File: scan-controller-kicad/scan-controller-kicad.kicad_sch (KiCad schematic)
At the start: 34 parts, among them CN1 24V in, J3 Raspi GPIO, J4 Raspi UART, J5 ICSP, J6 FTDI, Q6 IRLML2502, Q7 IRLML6402, SW6 Reset, U6 ATmega328P, Y1 8MHz

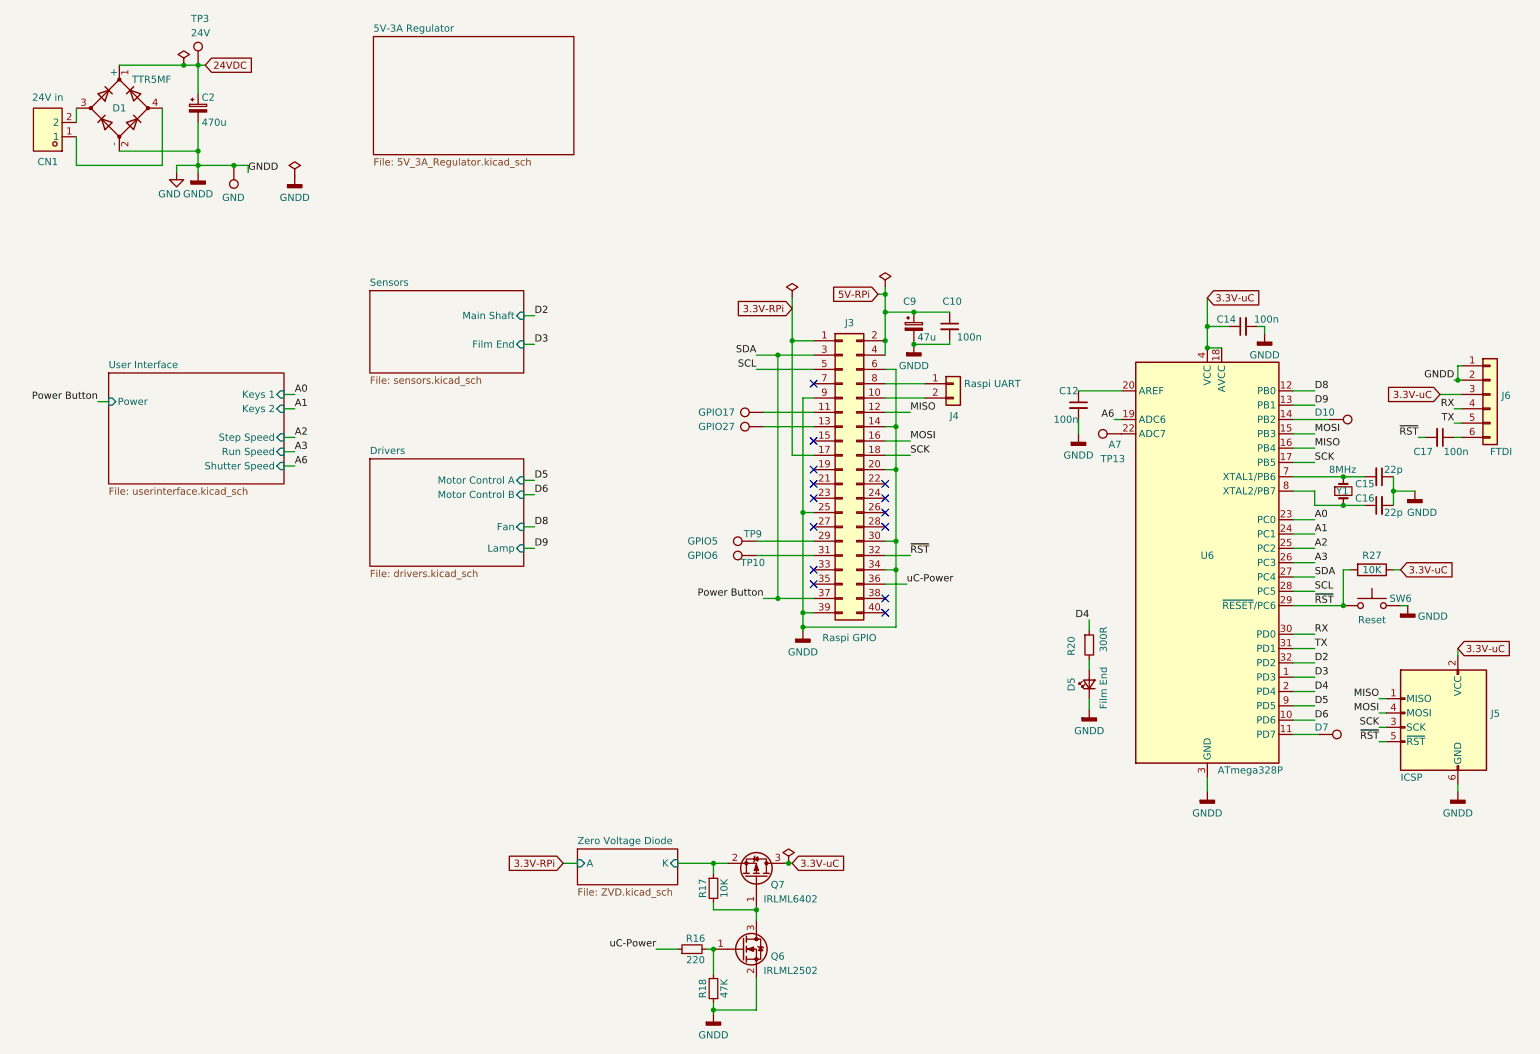
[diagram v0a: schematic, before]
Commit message: It's getting neat and readable
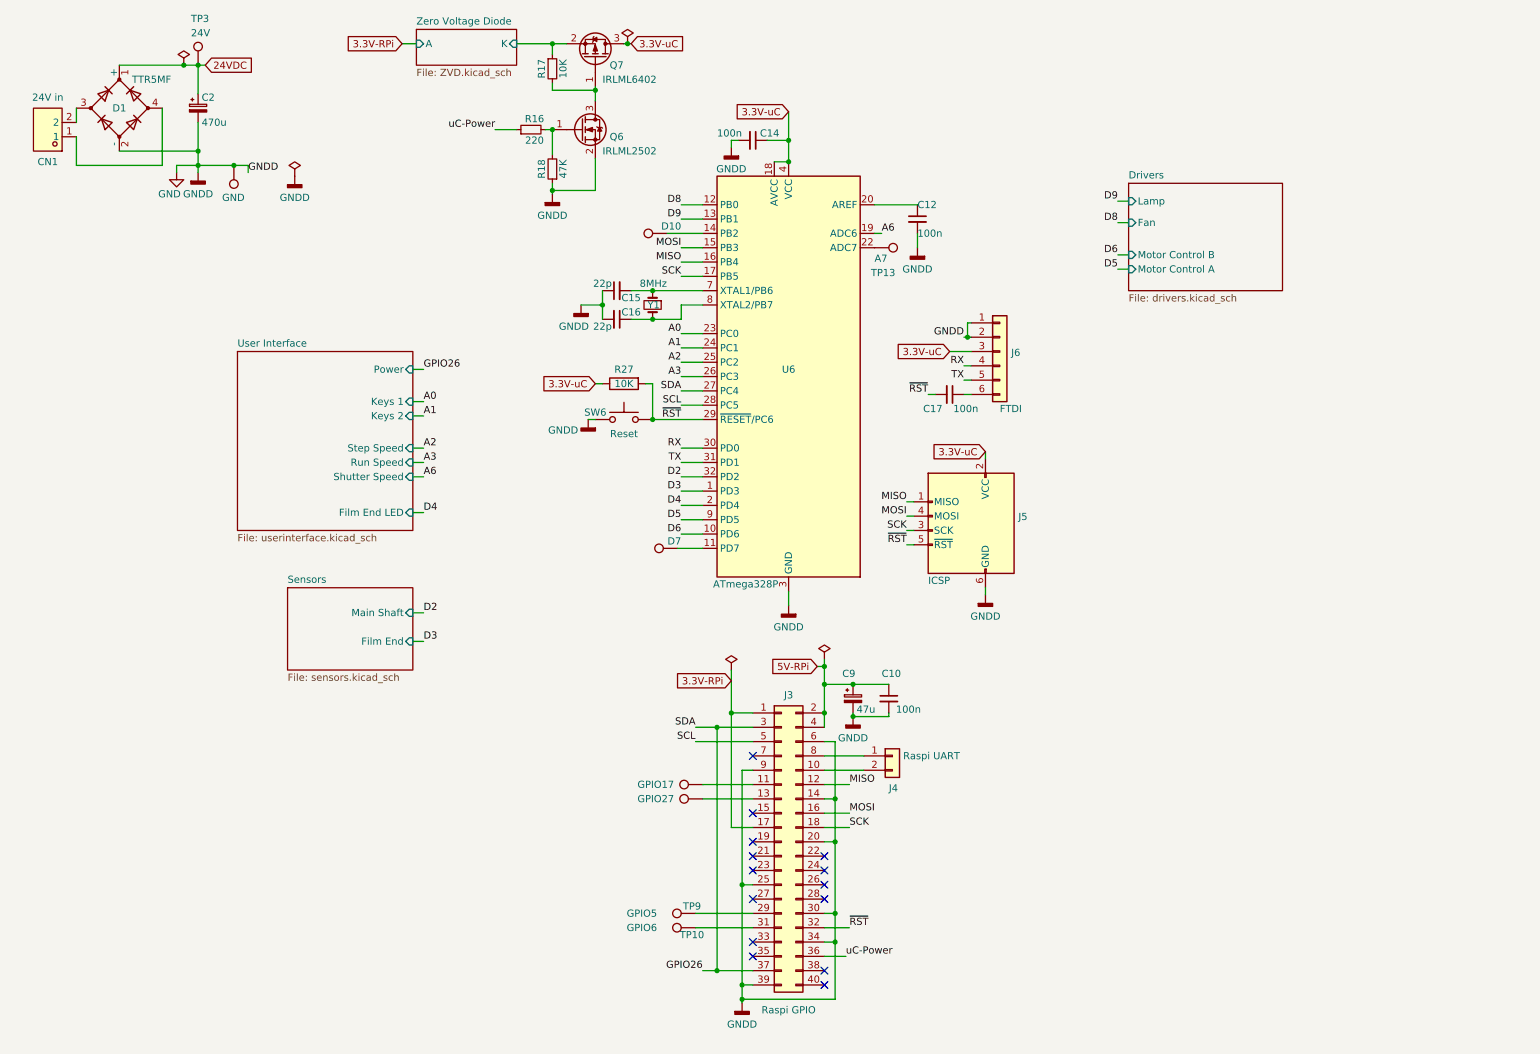
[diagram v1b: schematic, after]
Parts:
- removed D5: Film End, LED_SMD:LED_0805_2012Metric, symbol Device:LED_Small
- removed R20: 300R, Resistor_SMD:R_0805_2012Metric, symbol Device:R_Small
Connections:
- net Power Button renamed GPIO26
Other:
- removed sheet 5V-3A Regulator
- sheet User Interface ports: added Film End LED; removed none
- moved on the sheet: C10, C12, C14, C15, C16, C17, C9, J3, J4, J5, J6, Q6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
